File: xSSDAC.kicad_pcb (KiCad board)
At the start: 2 copper layers, 100 x 80 mm, 215 parts, among them J1 Conn_01x04, J2 ZX62-B-5PA_11, J3 625-7296, J4 Conn_01x08, J6 Micro_SD_Card_Det_Hirose_DM3AT, J8 RJ-2410N, J9 RJ-2410N, K1 UD2-5NUN, Q1 2SA1162-GR, Q2 2SA1162-GR, Q3 2SC2712-GR,LF, Q4 2SC2712-GR,LF, U1 XU216-512-TQ128-C20, U10 CDCLVC1103PWR, U11 SN74LVC1G79DBVR, U12 SN74LVC1G80DBVR, U13 SN74LVC1G02DBVR, U14 SN74LVC1G79DBVR, U15 SN74LVC1G80DBVR, U16 DAC8581IPW, U17 DAC8581IPW, U18 TAR5S25U(F), U19 MP1584EN-LF-Z, U2 MAU106, U20 MP1584EN-LF-Z, U21 NC7SZU04M5X, U22 SN74LVC1G02DBVR, U3 Si5351A-B-GT, U4 TL431PK, U5 TPD3E001DRLR, U6 IS25LP080D-JBLE, U7 NCP303LSN30T1G, U8 ADM1085AKSZ-REEL7, U9 NC7WZ07P6X, Y1 HC49S-24MHZ, Y2 FA-238_25.0000MB-K3

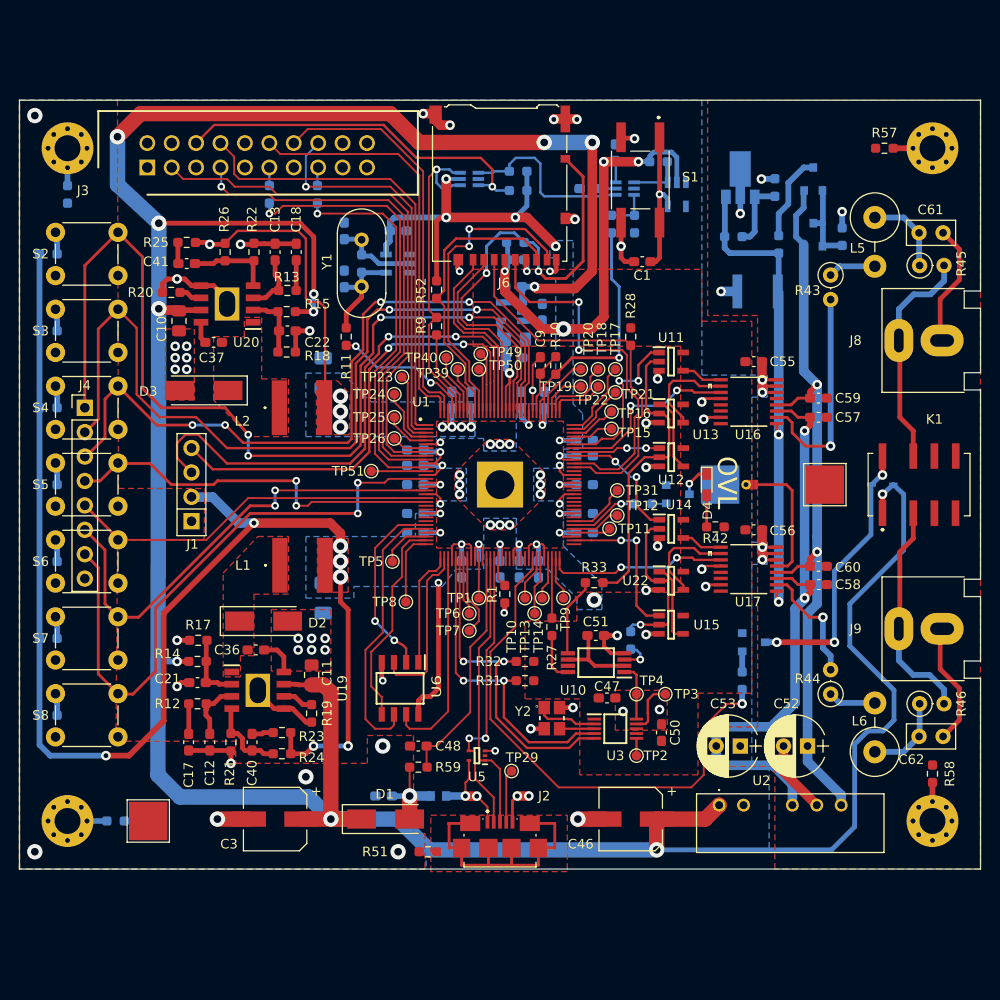
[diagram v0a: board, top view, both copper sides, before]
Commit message: V2.0
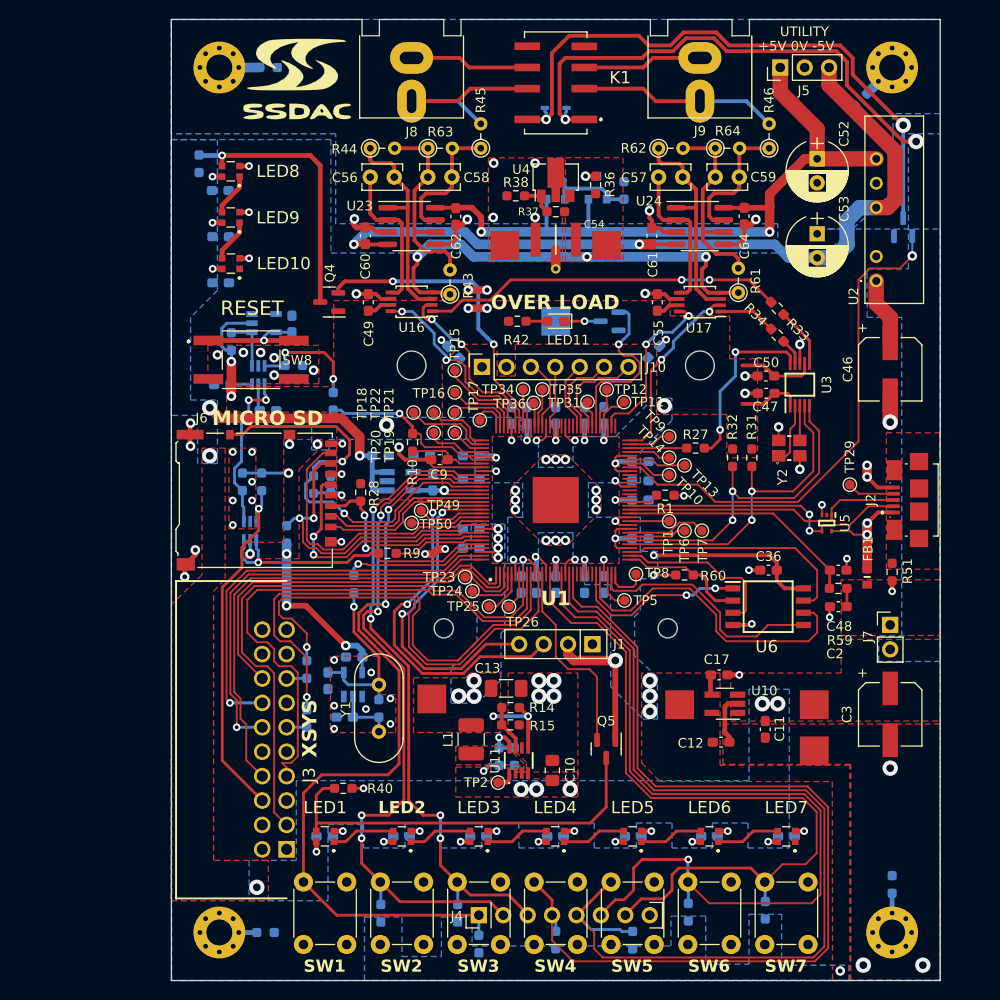
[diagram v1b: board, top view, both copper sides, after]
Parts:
- removed the C10 at (110.8, 81.4)
- removed the C13 at (120.8, 74.2)
- removed C41: 2.7n, Capacitor_SMD:C_0603_1608Metric_Pad1.08x0.95mm_HandSolder
- removed C43: 22u (1206), Capacitor_SMD:C_1206_3216Metric_Pad1.33x1.80mm_HandSolder
- removed C51: 100n, Capacitor_SMD:C_0603_1608Metric_Pad1.08x0.95mm_HandSolder
- removed D1, D2, D3: SJPA-D3, pretty:D_SJP_Handsoldering
- removed D4: LED, LEDs:LED_0603_HandSoldering
- removed L2: NR6028T4R7N, SamacSys_Parts:NR6020T2R2N
- removed L5, L6: AL0510 4.7mH, Inductors_THT:L_Axial_L12.0mm_D5.0mm_P5.08mm_Vertical_Fastron_MISC
- removed the R12 at (112.7, 121.2)
- removed the R14 at (112.7, 116.8)
- removed R17: 71.5k, Resistor_SMD:R_0603_1608Metric_Pad0.98x0.95mm_HandSolder
- removed R19: 190K, Resistor_SMD:R_0603_1608Metric_Pad0.98x0.95mm_HandSolder
- removed R21: 6.3k, Resistor_SMD:R_0603_1608Metric_Pad0.98x0.95mm_HandSolder
- removed R22: 80.6k, Resistor_SMD:R_0603_1608Metric_Pad0.98x0.95mm_HandSolder
- removed R23: 10.2k, Resistor_SMD:R_0603_1608Metric_Pad0.98x0.95mm_HandSolder
- removed R24: 20k, Resistor_SMD:R_0603_1608Metric_Pad0.98x0.95mm_HandSolder
- removed R25: 0, Resistor_SMD:R_0603_1608Metric_Pad0.98x0.95mm_HandSolder
- removed R26: 20K, Resistor_SMD:R_0603_1608Metric_Pad0.98x0.95mm_HandSolder
- removed R41: 0, pretty:BIND_PTH_NPTH
- removed TP39, TP40, TP51: TestPoint, pretty:TestPoint_Pad_D1.0mm_noCrtYd
- removed U12, U15: SN74LVC1G80DBVR, pretty:SOT95P280X145-5N
- removed U13, U22: SN74LVC1G02DBVR, pretty:SOT95P280X145-5N
- removed U14: SN74LVC1G79DBVR, pretty:SOT95P280X145-5N
- removed U19, U20: MP1584EN-LF-Z, pretty:SOIC127P600X170-9N
- added ART1: Silk Only, pretty:SSDACLOGO_190X190, F.Cu at (123.1, 56.0)
- added C11: 100n, Capacitor_SMD:C_0603_1608Metric_Pad1.08x0.95mm_HandSolder, F.Cu at (171.8, 123.9)
- added C55: 100n, Capacitor_SMD:C_0603_1608Metric_Pad1.08x0.95mm_HandSolder, F.Cu at (160.6, 79.4)
- added C64: 100n, Capacitor_SMD:C_0603_1608Metric_Pad1.08x0.95mm_HandSolder, F.Cu at (169.6, 70.5)
- added C65: 100n, Capacitor_SMD:C_0603_1608Metric_Pad1.08x0.95mm_HandSolder, B.Cu at (115.1, 67.8)
- added C66: 100n, Capacitor_SMD:C_0603_1608Metric_Pad1.08x0.95mm_HandSolder, B.Cu at (115.1, 72.6)
- added C67: 100n, Capacitor_SMD:C_0603_1608Metric_Pad1.08x0.95mm_HandSolder, B.Cu at (115.1, 77.4)
- added C68: 100n, Capacitor_SMD:C_0603_1608Metric_Pad1.08x0.95mm_HandSolder, B.Cu at (150.0, 135.0)
- added C69: 100n, Capacitor_SMD:C_0603_1608Metric_Pad1.08x0.95mm_HandSolder, B.Cu at (158.1, 135.0)
- added C70: 100n, Capacitor_SMD:C_0603_1608Metric_Pad1.08x0.95mm_HandSolder, B.Cu at (166.0, 135.0)
- added J10: PIN SOCKET 01x07, pretty:OLED_7pin_0.95_96X64_RGB, F.Cu at (150.0, 100.0)
- added J5: PIN HEADER 01x03, Connector_PinHeader_2.54mm:PinHeader_1x03_P2.54mm_Vertical, F.Cu at (173.4, 55.0)
- added J7: PIN HEADER 01x02, Connector_PinHeader_2.54mm:PinHeader_1x02_P2.54mm_Vertical, F.Cu at (184.8, 113.0)
- added LED1: WS2812C-2020, pretty:WS2812C2020, F.Cu at (126.0, 135.0)
- added LED10: WS2812C-2020, pretty:WS2812C2020, F.Cu at (116.2, 75.4)
- added LED11: LED(Red), LED_SMD:LED_0603_1608Metric_Pad1.05x0.95mm_HandSolder, F.Cu at (150.0, 81.4)
- added LED2: WS2812C-2020, pretty:WS2812C2020, F.Cu at (134.0, 135.0)
- added LED3: WS2812C-2020, pretty:WS2812C2020, F.Cu at (142.0, 135.0)
- added LED4: WS2812C-2020, pretty:WS2812C2020, F.Cu at (149.9, 135.0)
- added LED5: WS2812C-2020, pretty:WS2812C2020, F.Cu at (158.0, 135.0)
- added LED6: WS2812C-2020, pretty:WS2812C2020, F.Cu at (166.0, 135.0)
- added LED7: WS2812C-2020, pretty:WS2812C2020, F.Cu at (174.0, 135.0)
- added LED8: WS2812C-2020, pretty:WS2812C2020, F.Cu at (116.2, 65.8)
- added LED9: WS2812C-2020, pretty:WS2812C2020, F.Cu at (116.2, 70.6)
- added NT1: Net-tie, cupper only, pretty:NetTie-2_SMD_Pad1.0mm, F.Cu at (150.0, 75.0)
- added Q5: BSS138, Package_TO_SOT_SMD:SOT-23, F.Cu at (155.2, 125.9)
- added Q6: BSS138, Package_TO_SOT_SMD:SOT-23, B.Cu at (155.6, 81.4)
- added R60: 10K, Resistor_SMD:R_0603_1608Metric_Pad0.98x0.95mm_HandSolder, F.Cu at (163.4, 107.8)
- added R61: 10K, Resistor_THT:R_Axial_DIN0204_L3.6mm_D1.6mm_P2.54mm_Vertical, F.Cu at (169.0, 78.4)
- added R62: 5K, Resistor_THT:R_Axial_DIN0204_L3.6mm_D1.6mm_P2.54mm_Vertical, F.Cu at (160.7, 63.4)
- added R63: 10K, Resistor_THT:R_Axial_DIN0204_L3.6mm_D1.6mm_P2.54mm_Vertical, F.Cu at (136.7, 63.4)
- added R64: 10K, Resistor_THT:R_Axial_DIN0204_L3.6mm_D1.6mm_P2.54mm_Vertical, F.Cu at (166.6, 63.4)
- added TP32: TestPoint, pretty:TestPoint_Pad_3.0x3.0mm, F.Cu at (162.9, 121.3)
- added TP33: TestPoint, pretty:TestPoint_Pad_3.0x3.0mm, F.Cu at (137.1, 120.7)
- added TP34: TestPoint, pretty:TestPoint_Pad_D1.0mm_noCrtYd, F.Cu at (146.6, 88.5)
- added TP35: TestPoint, pretty:TestPoint_Pad_D1.0mm_noCrtYd, F.Cu at (148.6, 88.5)
- added TP36: TestPoint, pretty:TestPoint_Pad_D1.0mm_noCrtYd, F.Cu at (147.7, 89.9)
- added U23: OPA2277UA, Package_SO:SOIC-8_3.9x4.9mm_P1.27mm, F.Cu at (135.0, 71.5)
- added U24: OPA2277UA, Package_SO:SOIC-8_3.9x4.9mm_P1.27mm, F.Cu at (165.0, 71.5)
- C1, C21, C22, C37, R11, R52, R57, R58: moved to B.Cu
- C12: value 2p -> 330n
- C13: renamed from C44; value 33u (1206) -> 22u (1206); moved to F.Cu
- C17: value 560p -> 10n
- C18: value 1n -> 100n; moved to B.Cu
- C2, FB1, R34, R36, R37, R38: moved to F.Cu
- C40: value 560p -> 100n; moved to B.Cu
- C5: value 10n -> 100n
- C52, C53: value 16SEPC100M -> OS-CON 16SEPC100M
- C54: value 16MU106MC44532 -> PLMCAP 10uF 16V; moved to F.Cu
- C56, C57, C58, C59: value 100n -> TBD; footprint Capacitor_SMD:C_0603_1608Metric_Pad1.08x0.95mm_HandSolder -> Capacitor_THT:C_Rect_L4.0mm_W2.5mm_P2.50mm
- C61, C62: value 0.1uF -> 100n; footprint Capacitors_THT:C_Disc_D5.0mm_W2.5mm_P2.50mm -> Capacitor_SMD:C_0603_1608Metric_Pad1.08x0.95mm_HandSolder
- C7: value 1u -> 220n
- C8: value 10u (0805) -> 10n; footprint Capacitor_SMD:C_0805_2012Metric_Pad1.18x1.45mm_HandSolder -> Capacitor_SMD:C_0603_1608Metric_Pad1.08x0.95mm_HandSolder
- J1: value Conn_01x04 -> PIN SOCKET 01x04; footprint pretty:OLED_128X64 -> pretty:OLED_4pin_1.3_128X64
- J2: value ZX62-B-5PA_11 -> USB JACK ZX62-B-5PA_11
- J3: value 625-7296 -> BOX HEADER 02x10; footprint SamacSys_Parts:SHDR20W64P254_2X10_3305X860X930P -> SamacSys:SHDRRA20W66P254_2X10_3289X986X927P
- J4: value Conn_01x08 -> NO ASM
- J8, J9: value RJ-2410N -> RCA JACK RJ-2410N
- K1: value UD2-5NUN -> UD2-5NU; footprint pretty:UD25NUN -> SamacSys:UD25NUN
- L1: value NR6028T100M -> 0.47uH, 8.7A (1210); footprint SamacSys_Parts:NR6020T2R2N -> Inductor_SMD:L_1210_3225Metric_Pad1.42x2.65mm_HandSolder
- Q3: value 2SC2712-GR,LF -> BSS138; footprint TO_SOT_Packages_SMD:SC-59 -> Package_TO_SOT_SMD:SOT-23
- Q4: value 2SC2712-GR,LF -> BSS138; footprint TO_SOT_Packages_SMD:SC-59 -> Package_TO_SOT_SMD:SOT-23; moved to F.Cu
- R12: renamed from R15; moved to B.Cu
- R13: value 22k -> 100K; moved to B.Cu
- R14: renamed from R18; value 71.5k -> 24K
- R15: renamed from R20; value 190K -> 36K
- R39: value 4K7 -> 1K
- R40: value 4K7 -> 1K; moved to F.Cu
- R43: value 820 -> 10K; footprint Resistors_THT:R_Axial_DIN0207_L6.3mm_D2.5mm_P2.54mm_Vertical -> Resistor_THT:R_Axial_DIN0204_L3.6mm_D1.6mm_P2.54mm_Vertical
- R44: value 820 -> 5K; footprint Resistors_THT:R_Axial_DIN0207_L6.3mm_D2.5mm_P2.54mm_Vertical -> Resistor_THT:R_Axial_DIN0204_L3.6mm_D1.6mm_P2.54mm_Vertical
- R45, R46: footprint Resistors_THT:R_Axial_DIN0207_L6.3mm_D2.5mm_P2.54mm_Vertical -> Resistor_THT:R_Axial_DIN0204_L3.6mm_D1.6mm_P2.54mm_Vertical
- R8: value 0 -> 10K
- SW1: renamed from S2; value TS-0606 -> SPST
- SW2: renamed from S3; value TS-0606 -> SPST
- SW3: renamed from S4; value TS-0606 -> SPST
- SW4: renamed from S5; value TS-0606 -> SPST
- SW5: renamed from S6; value TS-0606 -> SPST
- SW6: renamed from S7; value TS-0606 -> SPST
- SW7: renamed from S8; value TS-0606 -> SPST
- TP2: value CLK2 -> TestPoint
- TP27, TP28, TP30: footprint TestPoint:TestPoint_Pad_4.0x4.0mm -> pretty:TestPoint_Pad_3.0x3.0mm
- TP3: value CLK1 -> TestPoint; footprint pretty:TestPoint_Pad_D1.0mm_noCrtYd -> pretty:TestPoint_Pad_3.0x3.0mm
- TP4: value CLK0 -> TestPoint; footprint pretty:TestPoint_Pad_D1.0mm_noCrtYd -> pretty:TestPoint_Pad_3.0x3.0mm
- U1: footprint pretty:QFP40P1600X1600X120-129N-D-TH -> pretty:QFP40P1600X1600X120-129N-D
- U10: value CDCLVC1103PWR -> NJM12877F33-TE1; footprint pretty:SOP65P640X120-8N -> Package_TO_SOT_SMD:SOT-23-5_HandSoldering
- U11: value SN74LVC1G79DBVR -> MPQ2172GJ-AEC1-Z; footprint pretty:SOT95P280X145-5N -> pretty:MPQ2172GJAEC1Z
- U16, U17: value DAC8581IPW -> DAC8811IBDGKT; footprint pretty:SOP65P640X120-16N -> Package_SO:TSSOP-8_3x3mm_P0.65mm
- U18: value TAR5S25U(F) -> NJM12877F25-TE1; footprint TO_SOT_Packages_SMD:SOT-23-5 -> Package_TO_SOT_SMD:SOT-23-5_HandSoldering
- U4: footprint pretty:PK_R-PSSO-F3_ -> Package_TO_SOT_SMD:SOT-89-3; moved to F.Cu
- U5: footprint SOTFL50P160X60-5N -> pretty:SOTFL50P160X60-5N
- U6: value IS25LP080D-JBLE -> S25FL132K0XMFI013; footprint pretty:SOIC127P600X175-8N -> SamacSys:SOIC127P800X216-8N
- moved H2 86.6 mm to (185.0, 145.0), turned to 90 degrees
- moved R29 84.6 mm to (142.0, 146.2), turned to 90 degrees
- moved H1 83.1 mm to (115.0, 145.0), turned to 90 degrees
- moved R56 81.1 mm to (185.0, 140.0), turned to 90 degrees
- moved R55 79.5 mm to (119.8, 145.0), turned to 0 degrees
- moved H4 78.5 mm to (185.0, 55.0), turned to 90 degrees
- moved R39 78.0 mm to (112.9, 65.0), turned to 90 degrees
- moved R54 77.3 mm to (171.8, 142.7), turned to 90 degrees
- moved SW7 75.7 mm to (174.0, 143.0), turned to -90 degrees
- moved H3 74.7 mm to (115.0, 55.0), turned to 90 degrees
- moved R44 74.3 mm to (130.7, 63.4), turned to 0 degrees
- moved SW1 72.9 mm to (126.0, 143.0), turned to -90 degrees
- moved C62 72.5 mm to (139.6, 70.5), turned to -90 degrees
- moved R50 72.4 mm to (158.0, 145.8), turned to 90 degrees
- moved R53 72.4 mm to (163.8, 142.9), turned to 90 degrees
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- renumbered C11 to C10, C55 to C49, S1 to SW8
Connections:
- C12 pad 1: Net-(C12-Pad1) -> +3V3
- C17 pad 1: Net-(C17-Pad1) -> Net-(U10-CS)
- C18 pad 1: Net-(C18-Pad1) -> GND
- C18 pad 2: GND -> +5V
- C21 pad 1: Net-(C21-Pad1) -> GND
- C21 pad 2: GND -> +5V
- C22 pad 1: Net-(C22-Pad1) -> GND
- C22 pad 2: GND -> +5V
- C35 pad 2: +2V5 -> +5V
- C36 pad 1: Net-(C36-Pad1) -> GND
- C36 pad 2: Net-(C36-Pad2) -> +3V3
- C37 pad 1: Net-(C37-Pad1) -> GND
- C37 pad 2: Net-(C37-Pad2) -> +3V3
- C40 pad 1: Net-(C40-Pad1) -> GND
- C40 pad 2: Net-(C40-Pad2) -> +3V3
- C5 pad 1: Net-(C5-Pad1) -> +5V
- C56 pad 1: GND -> Net-(U16-IOUT)
- C56 pad 2: +3V3 -> Net-(U16-RFB)
- C57 pad 1: VEE -> Net-(U17-IOUT)
- C57 pad 2: GNDA -> Net-(U17-RFB)
- C58 pad 1: VEE -> Net-(C58-Pad1)
- C58 pad 2: GNDA -> Net-(U23B--)
- C59 pad 1: VDD -> Net-(C59-Pad1)
- C59 pad 2: GNDA -> Net-(U24B--)
- C60 pad 1: VDD -> VEE
- C61 pad 1: Net-(C61-Pad1) -> VEE
- C62 pad 1: Net-(C62-Pad1) -> VDD
- C7 pad 1: +5V -> +2V5
- C8 pad 1: +2V5 -> Net-(U18-CS)
- J3 pad 10: Net-(J3-Pad10) -> unconnected-(J3-Pad10)
- J3 pad 18: Net-(J3-Pad18) -> unconnected-(J3-Pad18)
- J3 pad 19: Net-(J3-Pad19) -> unconnected-(J3-Pad19)
- J3 pad 2: Net-(J3-Pad2) -> unconnected-(J3-Pad2)
- J3 pad 20: Net-(J3-Pad20) -> unconnected-(J3-Pad20)
- J3 pad 4: Net-(J3-Pad4) -> unconnected-(J3-Pad4)
- J6 pad 3: X1D0 -> X1D11
- J6 pad 5: X1D1 -> X1D10
- K1 pad 4: Net-(K1-Pad4) -> unconnected-(K1-NO_1-Pad4)
- K1 pad 5: Net-(K1-Pad5) -> unconnected-(K1-NO_2-Pad5)
- L1 pad 1: Net-(C36-Pad2) -> Net-(U11-SW)
- L1 pad 2: +3V3 -> +1V0
- Q3 pad 1: Net-(Q3-Pad1) -> X0D14
- Q4 pad 1: Net-(Q4-Pad1) -> +3V3
- Q4 pad 2: GND -> X0D25
- Q4 pad 3: Net-(D4-Pad1) -> Net-(LED8-DI)
- R12 pad 2: Net-(C22-Pad1) -> Net-(U11-EN)
- R13 pad 1: Net-(C18-Pad1) -> GND
- R13 pad 2: Net-(C13-Pad1) -> Net-(U11-EN)
- R14 pad 1: Net-(C22-Pad1) -> +1V0
- R14 pad 2: GND -> Net-(U11-FB)
- R15 pad 2: Net-(R20-Pad2) -> Net-(U11-FB)
- R27 pad 1: Net-(R27-Pad1) -> Net-(U3-CLK0)
- R28 pad 2: X1D0 -> X1D11
- R29 pad 2: Net-(R29-Pad2) -> X1D42
- R30 pad 2: Net-(R30-Pad2) -> X1D41
- R33 pad 2: Net-(R33-Pad2) -> Net-(U3-CLK2)
- R34 pad 2: Net-(R34-Pad2) -> Net-(U3-CLK1)
- R39 pad 1: Net-(Q3-Pad1) -> +5V
- R39 pad 2: X0D14 -> Net-(LED8-DI)
- R40 pad 1: Net-(Q4-Pad1) -> +5V
- R40 pad 2: X0D18 -> Net-(LED1-DI)
- R43 pad 1: Net-(L5-Pad2) -> /SerialDAC/VREF
- R43 pad 2: Net-(R43-Pad2) -> Net-(U23B--)
- R44 pad 1: Net-(L6-Pad2) -> Net-(U16-RFB)
- R44 pad 2: Net-(R44-Pad2) -> Net-(U23B--)
- R45 pad 1: Net-(C61-Pad1) -> Net-(C58-Pad1)
- R46 pad 1: Net-(C62-Pad1) -> Net-(C59-Pad1)
- R48 pad 2: Net-(R48-Pad2) -> X1D40
- R49 pad 2: Net-(R49-Pad2) -> X1D39
- R50 pad 2: Net-(R50-Pad2) -> X1D38
- R53 pad 2: Net-(R53-Pad2) -> X1D37
- R54 pad 2: Net-(R54-Pad2) -> X1D36
- SW1 pad 3: Net-(R29-Pad2) -> unconnected-(SW1-Pad3)
- SW2 pad 3: Net-(R30-Pad2) -> unconnected-(SW2-Pad3)
- SW3 pad 3: Net-(R48-Pad2) -> unconnected-(SW3-Pad3)
- SW4 pad 3: Net-(R49-Pad2) -> unconnected-(SW4-Pad3)
- SW5 pad 3: Net-(R50-Pad2) -> unconnected-(SW5-Pad3)
- SW6 pad 3: Net-(R53-Pad2) -> unconnected-(SW6-Pad3)
- SW7 pad 3: Net-(R54-Pad2) -> unconnected-(SW7-Pad3)
- TP2 pad 1: Net-(TP2-Pad1) -> Net-(U11-PG)
- TP3 pad 1: Net-(TP3-Pad1) -> /SerialDAC/VREF
- TP4 pad 1: Net-(TP4-Pad1) -> +5V
- U1 pad 50: Net-(U1-Pad50) -> unconnected-(U1-NC_1-Pad50)
- U1 pad 65: Net-(U1-Pad65) -> unconnected-(U1-NC_2-Pad65)
- U10 pad 1: Net-(TP4-Pad1) -> +5V
- U10 pad 2: +3V3 -> GND
- U10 pad 3: Net-(R34-Pad2) -> +5V
- U10 pad 4: GND -> Net-(U10-CS)
- U10 pad 5: Net-(R33-Pad2) -> +3V3
- U11 pad 1: X0D35 -> Net-(U11-PG)
- U11 pad 2: /SerialDAC/CLK_DACL -> +5V
- U11 pad 3: GND -> Net-(U11-SW)
- U11 pad 4: /SerialDAC/SDIN-L -> GND
- U11 pad 5: +3V3 -> +1V0
- U16 pad 1: /SerialDAC/VREF -> /SerialDAC/CLK_DACL
- U16 pad 2: Net-(R43-Pad2) -> X0D34
- U16 pad 3: VEE -> Net-(U16-RFB)
- U16 pad 4: VDD -> /SerialDAC/VREF
- U16 pad 5: GNDA -> Net-(U16-IOUT)
- U16 pad 7: GND -> +3V3
- U16 pad 8: GND -> X0D35
- U17 pad 1: /SerialDAC/VREF -> /SerialDAC/CLK_DACR
- U17 pad 2: Net-(R44-Pad2) -> X0D22
- U17 pad 3: VEE -> Net-(U17-RFB)
- U17 pad 4: VDD -> /SerialDAC/VREF
- U17 pad 5: GNDA -> Net-(U17-IOUT)
- U17 pad 7: GND -> +3V3
- U17 pad 8: GND -> X0D23
- U18 pad 3: Net-(C5-Pad1) -> +5V
- U18 pad 4: +2V5 -> Net-(U18-CS)
- U18 pad 5: +5V -> +2V5
- U21 pad 1: Net-(U21-Pad1) -> unconnected-(U21-NC-Pad1)
- U3 pad 10: Net-(TP4-Pad1) -> Net-(U3-CLK0)
- U3 pad 6: Net-(TP2-Pad1) -> Net-(U3-CLK2)
- U3 pad 9: Net-(TP3-Pad1) -> Net-(U3-CLK1)
- U5 pad 2: Net-(U5-Pad2) -> unconnected-(U5-IO2-Pad2)
- U6 pad 1: X0D5 -> X0D1
- U6 pad 2: X0D1 -> X0D5
- U7 pad 4: Net-(U7-Pad4) -> unconnected-(U7-NC-Pad4)
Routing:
- net +5V: track 338.2 -> 101.0 mm, vias 12 -> 23
- net +3V3: track 283.3 -> 127.1 mm, vias 28 -> 31
- net X1D38: track 38.9 -> 100.7 mm
- net X1D39: track 40.1 -> 99.1 mm, vias 2 -> 0
- net Net-(LED1-DI): track 0.00 -> 41.9 mm
- net GND: track 118.8 -> 79.6 mm, vias 72 -> 81
- net X1D37: track 49.0 -> 87.7 mm, vias 2 -> 1
- net X1D1: track 38.1 -> 2.44 mm, vias 2 -> 0
- net X1D0: track 39.5 -> 3.97 mm
- net Net-(K1-COIL_-): track 28.7 -> 63.4 mm, vias 3 -> 2
- net +1V0: track 110.2 -> 76.8 mm, vias 19 -> 20
- net Net-(LED8-DI): track 0.00 -> 28.5 mm, vias 0 -> 1
- net /xCORE/FG: track 28.2 -> 0.00 mm
- net Net-(U17-RFB): track 0.00 -> 24.4 mm
- net VEE: track 62.8 -> 86.3 mm
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- added copper zone on B.Cu, net +5V
- added copper zone on F.Cu, net +5V
- added copper zone on F.Cu, net /SerialDAC/VREF
- added copper zone on B.Cu, net GNDA
- added copper zone on F.Cu, net Net-(J7-Pin_1)
- added copper zone on F.Cu, net Net-(U11-SW)
- removed copper zone on F.Cu, net Net-(C36-Pad2)
- removed copper zone on F.Cu, net Net-(C37-Pad2)
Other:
- board size 100 x 80 mm -> 80 x 100 mm
- board text added: "+5V 0V -5V"
- board text added: "MICRO SD"
- board text added: "OVER LOAD"
- board text added: "RESET"
- board text added: "UTILITY"
- board text added: "XSYS"
- board text added: "xSSDAC SD player v2.0 T. Sakurai Aug 2023"
- board text removed: "OVL"
- board text removed: "xSSDAC SD player v1.0 T. Sakurai May 2021"
